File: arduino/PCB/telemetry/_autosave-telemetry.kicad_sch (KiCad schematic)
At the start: 1 part, among them U1 ATmega2560-16A

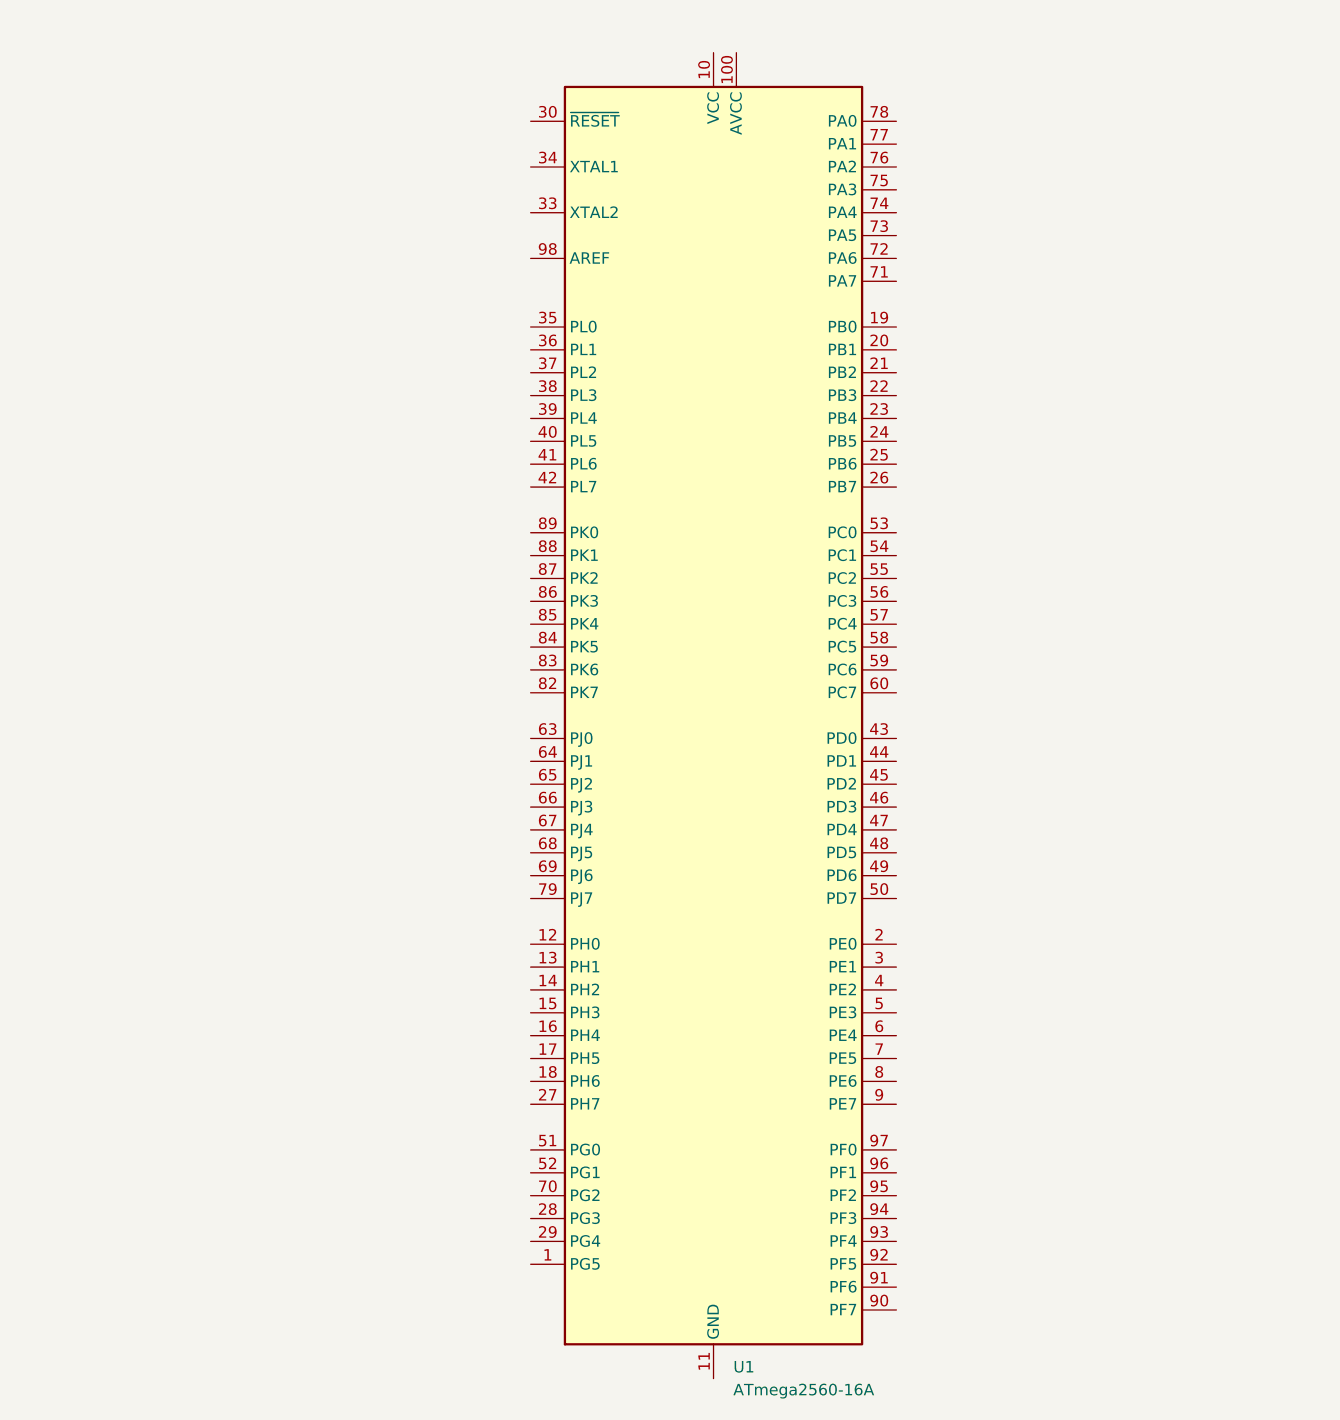
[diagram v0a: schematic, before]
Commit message: Agregando objeto laps
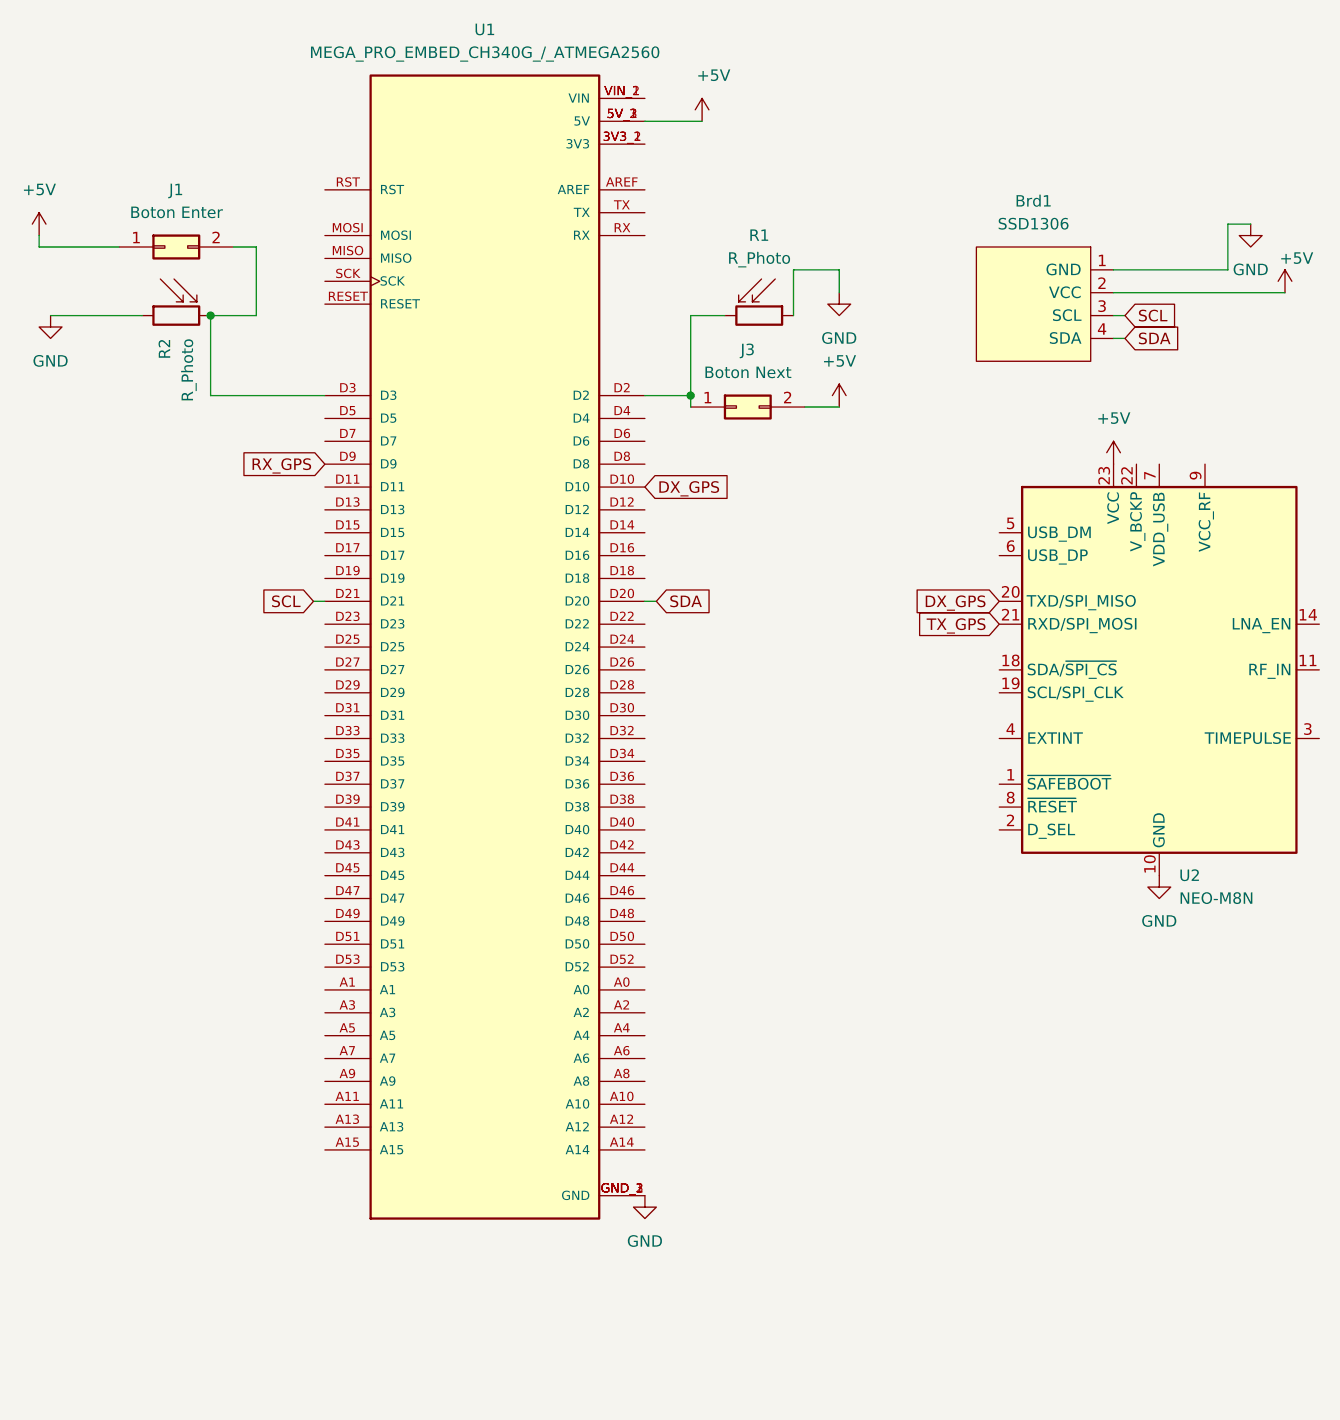
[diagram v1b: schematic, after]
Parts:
- removed U1: ATmega2560-16A, Package_QFP:TQFP-100_14x14mm_P0.5mm, symbol MCU_Microchip_ATmega:ATmega2560-16A
- added Brd1: SSD1306, SSD1306:128x64OLED, symbol SSD1306-128x64_OLED:SSD1306
- added J1: Boton Enter, Button_Switch_SMD:SW_SPST_EVPBF, symbol Connector_Generic:Conn_02x01
- added J3: Boton Next, Button_Switch_SMD:SW_SPST_EVPBF, symbol Connector_Generic:Conn_02x01
- added R1, R2: R_Photo, Resistor_THT:R_Axial_DIN0204_L3.6mm_D1.6mm_P7.62mm_Horizontal, symbol Device:R_Photo
- added U1: MEGA_PRO_EMBED_CH340G_/_ATMEGA2560, MEGA_PRO_EMBED_CH340G___ATMEGA2560:MODULE_MEGA_PRO_EMBED_CH340G___ATMEGA2560, symbol MEGA_PRO_EMBED_CH340G___ATMEGA2560:MEGA_PRO_EMBED_CH340G_/_ATMEGA2560
- added U2: NEO-M8N, Sensor:Aosong_DHT11_5.5x12.0_P2.54mm, symbol RF_GPS:NEO-M8N
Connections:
- new net: J3.1 (Pin_1), R1.2, U1.D2
- new net: U1.3V3_1 (3V3), U1.3V3_2 (3V3)
- new net: J1.2 (Pin_2), R2.2, U1.D3
- new net: U1.VIN_1 (VIN), U1.VIN_2 (VIN)
- new net +5V: Brd1.2 (VCC), J1.1 (Pin_1), J3.2 (Pin_2), U1.5V_1 (5V), U1.5V_2 (5V), U1.5V_3 (5V), U2.23 (VCC)
- new net DX_GPS: U1.D10, U2.20 (TXD/SPI_MISO)
- new net GND: Brd1.1 (GND), R1.1, R2.1, U1.GND_1 (GND), U1.GND_2 (GND), U1.GND_3 (GND), U2.10 (GND), U2.12 (GND), U2.13 (GND), U2.24 (GND)
- new net RX_GPS: U1.D9
- new net SCL: Brd1.3 (SCL), U1.D21
- new net SDA: Brd1.4 (SDA), U1.D20
- new net TX_GPS: U2.21 (RXD/SPI_MOSI)
